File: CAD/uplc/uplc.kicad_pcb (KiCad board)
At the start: 4 copper layers, 31.2 x 20.5 mm, 46 parts, among them J1 Conn_01x06_Pin, J2 SM12B-GHS-TB(LF)(SN), K1 G6K-2F-Y, K2 G6K-2F-Y, U1 DS8242-33S5, U3 ESP32-C3-WROOM-02, U5 TBD62003AFWG, Y1 32.568khz

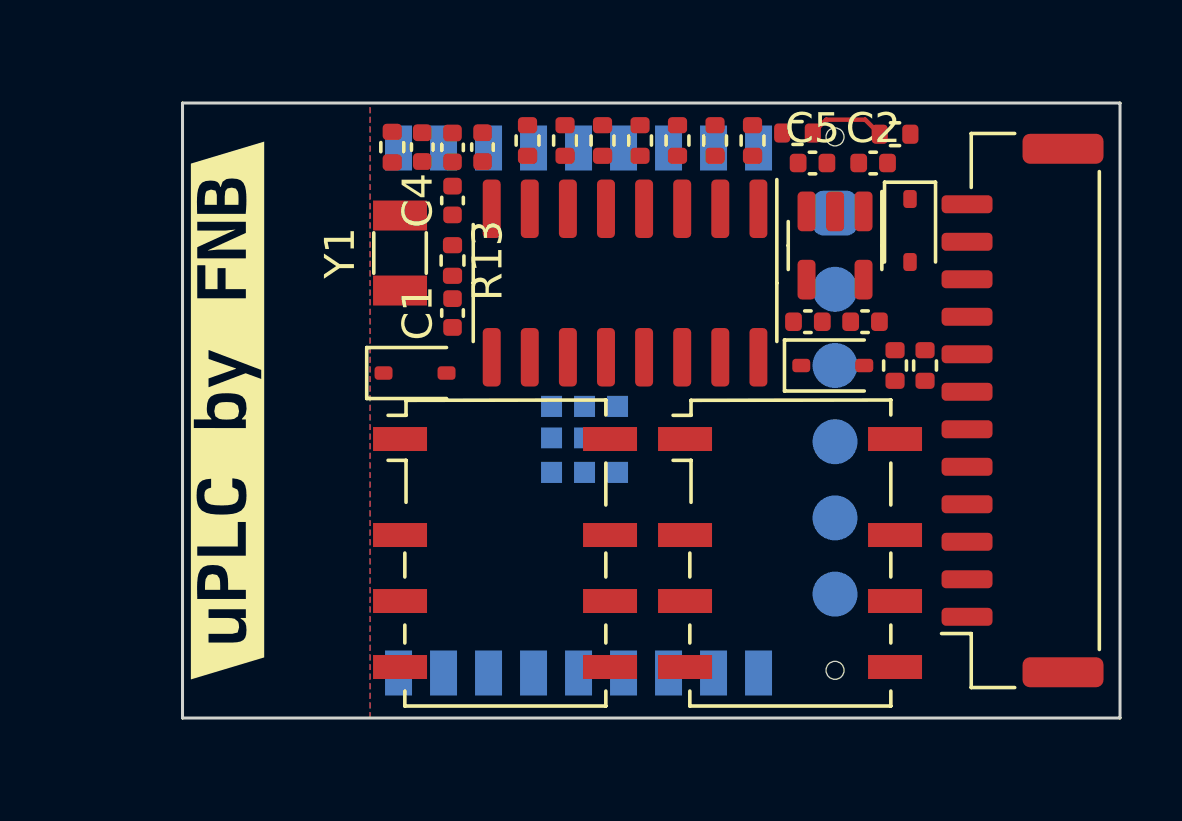
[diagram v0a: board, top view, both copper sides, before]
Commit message: wip
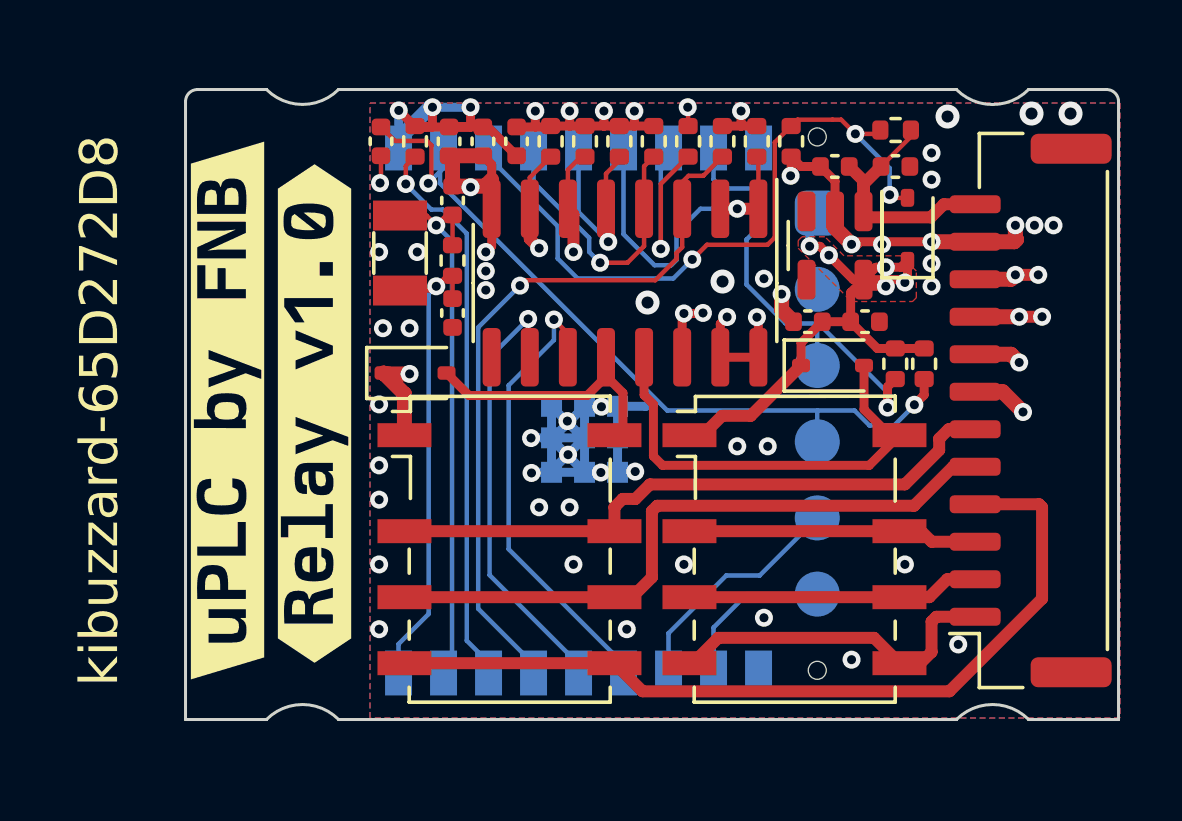
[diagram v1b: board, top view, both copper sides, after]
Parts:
- removed the D2 at (124.2, 76.5)
- removed kibuzzard-65666C6B: G***, esprelay:kibuzzard-65666C6B
- removed kibuzzard-65666C71: G***, esprelay:kibuzzard-65666C71
- removed kibuzzard-65666C76: G***, esprelay:kibuzzard-65666C76
- removed kibuzzard-65666C7B: G***, esprelay:kibuzzard-65666C7B
- removed kibuzzard-65666C87: G***, esprelay:kibuzzard-65666C87
- removed kibuzzard-65666CB7: G***, esprelay:kibuzzard-65666CB7
- removed kibuzzard-65CFDA91: G***, esprelay:kibuzzard-65CFDA91
- removed kibuzzard-65CFDAA0: G***, esprelay:kibuzzard-65CFDAA0
- removed kibuzzard-65CFDAA7: G***, esprelay:kibuzzard-65CFDAA7
- removed kibuzzard-65CFDAAD: G***, esprelay:kibuzzard-65CFDAAD
- removed kibuzzard-65CFDAB5: G***, esprelay:kibuzzard-65CFDAB5
- removed kibuzzard-65CFDABC: G***, esprelay:kibuzzard-65CFDABC
- added C6: 0.1uF, Capacitor_SMD:C_0402_1005Metric, F.Cu at (106.6, 73.5)
- added D3: 1N5819WS, Diode_SMD:D_SOD-323, F.Cu at (124.2, 76.5)
- added kibuzzard-65D3605C: G***, kibuzzard-65D3605C, F.Cu at (104.4, 82.6)
- added kibuzzard-65D3616E: G***, kibuzzard-65D3616E, B.Cu at (128.0, 74.0)
- added kibuzzard-65D36177: G***, kibuzzard-65D36177, B.Cu at (128.0, 75.6)
- added kibuzzard-65D3619D: G***, kibuzzard-65D3619D, B.Cu at (128.0, 78.7)
- added kibuzzard-65D361A7: G***, kibuzzard-65D361A7, B.Cu at (128.0, 77.1)
- added kibuzzard-65D361B0: G***, kibuzzard-65D361B0, B.Cu at (128.0, 80.2)
- added kibuzzard-65D361D3: G***, kibuzzard-65D361D3, B.Cu at (128.0, 81.8)
- added kibuzzard-65D361E1: G***, kibuzzard-65D361E1, B.Cu at (128.0, 83.3)
- added kibuzzard-65D361E9: G***, kibuzzard-65D361E9, B.Cu at (128.0, 84.9)
- added kibuzzard-65D361F2: G***, kibuzzard-65D361F2, B.Cu at (128.0, 86.4)
- added kibuzzard-65D361FD: G***, kibuzzard-65D361FD, B.Cu at (128.0, 88.0)
- added kibuzzard-65D36206: G***, kibuzzard-65D36206, B.Cu at (128.0, 89.5)
- added kibuzzard-65D3620E: G***, kibuzzard-65D3620E, B.Cu at (128.0, 91.1)
- added kibuzzard-65D36263: G***, kibuzzard-65D36263, B.Cu at (123.5, 86.1)
- added kibuzzard-65D36263: G***, kibuzzard-65D36263, B.Cu at (123.6, 78.4)
- added kibuzzard-65D36263: G***, kibuzzard-65D36263, B.Cu at (123.5, 75.9)
- added kibuzzard-65D36263: G***, kibuzzard-65D36263, B.Cu at (123.6, 83.5)
- added kibuzzard-65D36263: G***, kibuzzard-65D36263, B.Cu at (123.5, 88.6)
- added kibuzzard-65D36263: G***, kibuzzard-65D36263, B.Cu at (123.7, 81.0)
- C1, C4: value 10pf -> 20pf
- D1, D2: value 1N4148WS -> 1N5819WS
- moved C3 1.15 mm to (111.1, 73.5), turned to 90 degrees
- moved C10 1.03 mm to (110.0, 73.5)
- moved R2 0.99 mm to (123.8, 80.9)
- moved R1 0.97 mm to (124.7, 80.9)
- moved C11 0.92 mm to (108.9, 73.5)
- moved R5 0.78 mm to (107.8, 73.5)
- moved R11 0.77 mm to (112.3, 73.5)
- moved C2 0.75 mm to (123.8, 74.4)
- moved C5 0.75 mm to (121.7, 74.4)
- moved R12 0.67 mm to (113.4, 73.5)
- moved J1 0.59 mm to (121.2, 75.9)
- moved R10 0.56 mm to (114.6, 73.5)
- moved R9 0.46 mm to (115.7, 73.5)
- moved R4 0.35 mm to (116.9, 73.5)
- moved R3 0.35 mm to (120.3, 73.5), turned to -90 degrees
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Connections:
- J1 pad 2: TX -> GND
- J1 pad 3: RX -> BOOT
- J1 pad 4: BOOT -> RST
- J1 pad 5: RST -> TX
- J1 pad 6: GND -> RX
- J2 pad 1: +VDC -> R2NO
- J2 pad 10: R2NC -> HO1
- J2 pad 11: R2CO -> GND
- J2 pad 12: R2NO -> +VDC
- J2 pad 2: GND -> R2CO
- J2 pad 3: HI1 -> R2NC
- J2 pad 4: HI2 -> R1NO
- J2 pad 5: HO1 -> R1CO
- J2 pad 6: HO2 -> R1NC
- J2 pad 7: R1NC -> HI2
- J2 pad 8: R1CO -> HI1
- J2 pad 9: R1NO -> HO2
- R10 pad 1: GPIO15 -> LI5
- R7 pad 1: GPIO13 -> LI12
- R8 pad 1: GPIO12 -> LI3
- R9 pad 1: GPIO14 -> LI4
- U3 pad 10: GPIO15 -> unconnected-(U3-GPIO10-Pad10)
- U3 pad 13: unconnected-(U3-GPIO18/USB_D--Pad13) -> LO6
- U3 pad 14: GPIO4 -> LO7
- U3 pad 15: ADC -> LI3
- U3 pad 3: GPIO5 -> ADC
- U3 pad 4: GPIO12 -> LI4
- U3 pad 5: GPIO13 -> LI5
- U3 pad 6: GPIO14 -> LI12
- U5 pad 1: GPIO13 -> LI12
- U5 pad 10: GPIO5 -> LO7
- U5 pad 11: GPIO4 -> LO6
- U5 pad 12: RO2 -> RO1
- U5 pad 13: RO1 -> RO2
- U5 pad 2: GPIO13 -> LI12
- U5 pad 3: GPIO12 -> LI3
- U5 pad 4: GPIO14 -> LI4
- U5 pad 5: GPIO15 -> LI5
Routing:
- net +3.3V: track 0.00 -> 63.7 mm, vias 0 -> 10
- net GND: track 0.00 -> 50.1 mm, vias 0 -> 55
- net R1NO: track 0.00 -> 28.5 mm
- net RST: track 0.00 -> 27.3 mm, vias 0 -> 2
- net LI3: track 0.00 -> 24.2 mm, vias 0 -> 1
- net HI2: track 0.00 -> 24.1 mm, vias 0 -> 2
- net HI1: track 0.00 -> 22.0 mm, vias 0 -> 2
- net R1CO: track 0.00 -> 21.8 mm
- net R1NC: track 0.00 -> 21.1 mm
- net ADC: track 2.62 -> 23.1 mm, vias 0 -> 3
- net Net-(U3-GPIO2/ADC1_CH2): track 0.00 -> 18.7 mm, vias 0 -> 1
- net Net-(U3-GPIO1/ADC1_CH1/XTAL_32K_N): track 0.00 -> 18.3 mm, vias 0 -> 1
- net HO2: track 0.00 -> 17.1 mm, vias 0 -> 4
- net HO1: track 0.00 -> 16.6 mm, vias 0 -> 4
- net Net-(U3-GPIO0/ADC1_CH0/XTAL_32K_P): track 0.00 -> 16.1 mm, vias 0 -> 1
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- added copper zone on F.Cu, net +3.3V
- added copper zone on In2.Cu, net +3.3V
- added copper zone on In1.Cu, net GND
- added copper zone on In2.Cu, net GND
- added copper zone on In2.Cu, net HO1
- added copper zone on In2.Cu, net HO2
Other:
- board size 31.2 x 20.5 mm -> 31.1 x 21 mm
